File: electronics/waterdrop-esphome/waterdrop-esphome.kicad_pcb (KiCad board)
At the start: 4 copper layers, 105 x 80 mm, 38 parts, among them J1 12V_IN, J2 12V_OUT, J3 Comm_RO, J4 Comm_Faucet, J5 Valve, K1 G5LE-1, Q1 BC817, U1 LM2596DS-ADJ, U2 ESP32-S3-Tiny, U3 74AHCT125, U4 TB67H450A

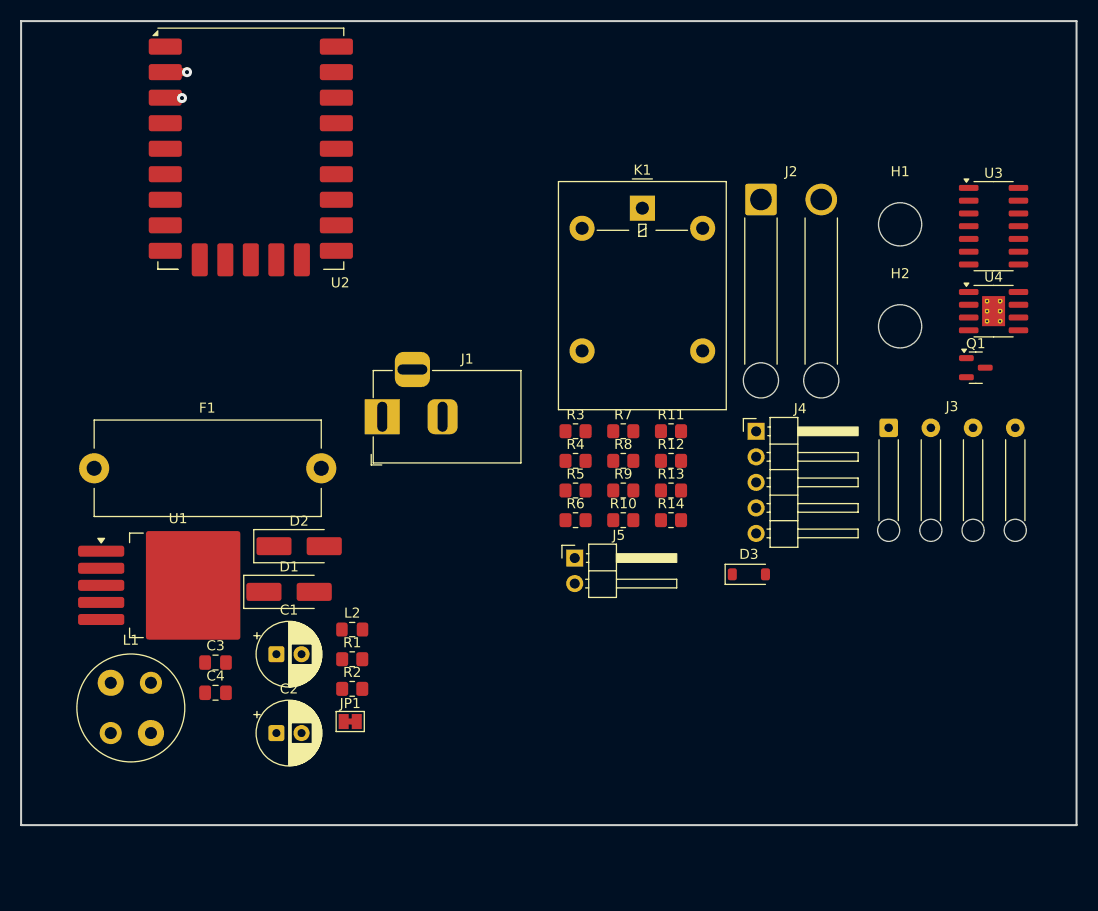
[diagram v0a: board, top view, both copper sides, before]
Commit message: PCB: lay out components
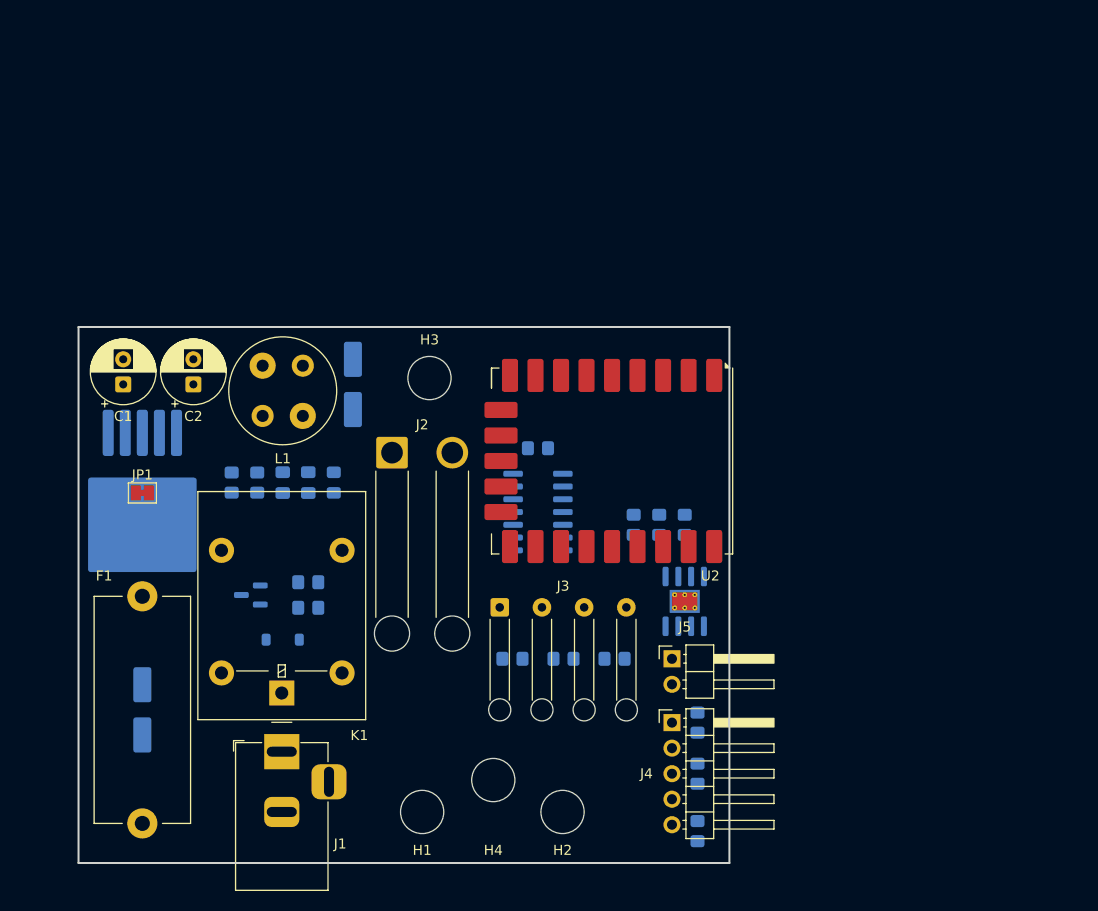
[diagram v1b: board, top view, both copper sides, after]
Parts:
- added H3: MountingHole, MountingHole:MountingHole_4.3mm_M4, F.Cu at (142.2, 86.3)
- added H4: MountingHole, MountingHole:MountingHole_4.3mm_M4, F.Cu at (148.6, 126.3)
- C3, C4, D1, D2, D3, L2, Q1, R1, R10, R11, R12, R13, R14, R2, R3, R4, R5, R6, R7, R8, R9, U1, U3, U4: moved to B.Cu
- H1, H2: footprint MountingHole:MountingHole_4.3mm_M4 -> MountingHole_extra:MountingHole_4.3mm
- moved Q1 75.6 mm to (124.5, 107.9), turned to 180 degrees
- moved H1 75.4 mm to (141.5, 129.5)
- moved K1 60.1 mm to (127.5, 117.7), turned to 180 degrees
- moved H2 58.9 mm to (155.5, 129.5)
- moved U3 53.5 mm to (153.0, 99.7)
- moved U2 47.5 mm to (160.4, 94.6), turned to -90 degrees
- moved D3 46.8 mm to (127.6, 112.4), turned to 180 degrees
- moved J2 44.5 mm to (138.5, 93.7)
- moved J3 42.6 mm to (149.2, 109.1)
- moved U4 42.2 mm to (167.6, 108.5), turned to -90 degrees
- moved C2 35.7 mm to (118.7, 87.0), turned to 90 degrees
- moved F1 35.7 mm to (113.7, 130.6), turned to 90 degrees
- moved J1 34.8 mm to (127.5, 123.5), turned to 90 degrees
- moved R9 34.7 mm to (168.9, 131.4), turned to -90 degrees
- moved L1 32.7 mm to (129.6, 90.1), turned to 180 degrees
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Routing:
- net GND: track 1.27 -> 0.00 mm, vias 1 -> 0
- net +3.3V: track 0.79 -> 0.00 mm, vias 1 -> 0
- removed copper zone on In2.Cu, net GND
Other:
- board size 105 x 80 mm -> 64.8 x 53.3 mm
